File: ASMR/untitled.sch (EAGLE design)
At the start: 60 parts, among them J1 U.FL-R-SMT(01), J3 2172034-1, J4 POWER_JACKSLT, Q1 MMBT3904, Q2 MMBT3904, Q3 12MHz, Q4 MC-306, U2 DS1307Z+, U3 MAX3444EASA, U4 AMS1117, U5 MAX232CSE, X1 MSTBA2

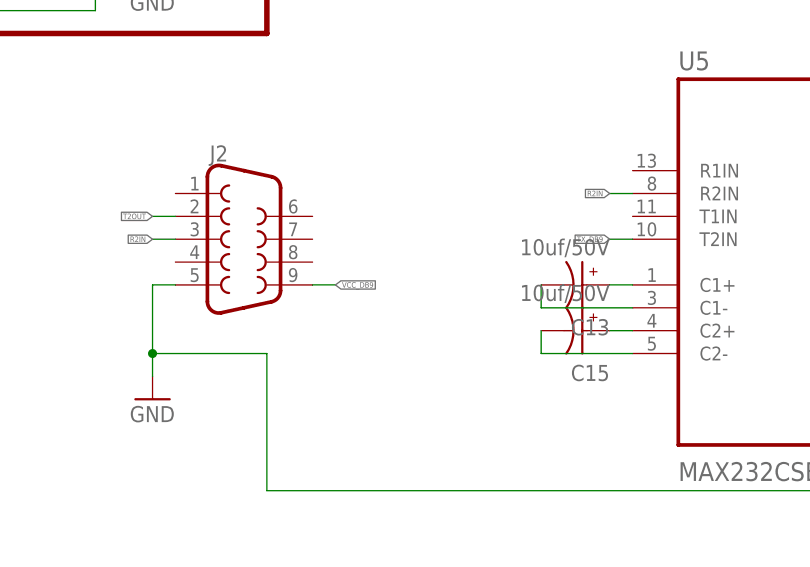
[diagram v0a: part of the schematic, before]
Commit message: penambahan komponen
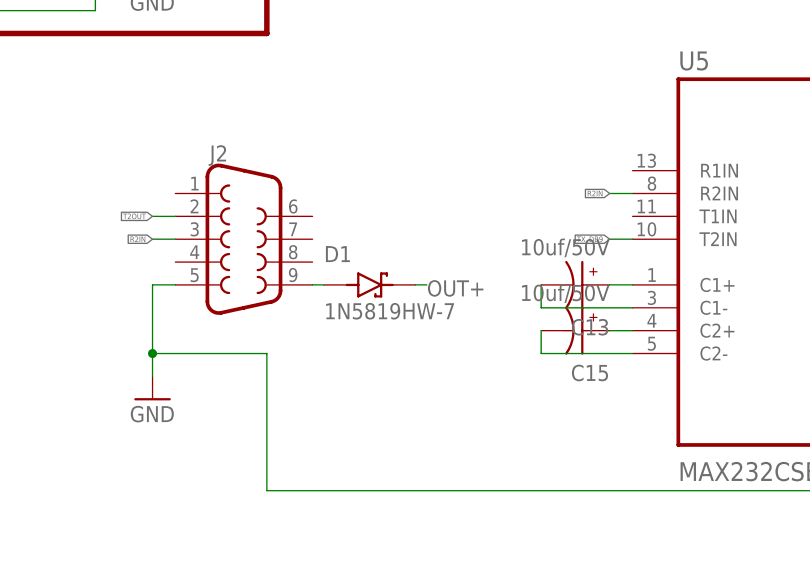
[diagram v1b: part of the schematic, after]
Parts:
- added D1: 1N5819HW-7, 1N5819HW-7:1N5819HW-7
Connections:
- new net N$20: D1.A, J2.9
- net OUT+: now also D1.K
- net VCC_DB9: no longer J2.9
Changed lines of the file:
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@@
 <part name="J1" library="U.FL-R-SMT_01_" deviceset="U.FL-R-SMT(01)" device=""/>
 <part name="JP3" library="pinhead" library_urn="urn:adsk.eagle:library:325" deviceset="PINHD-1X3" device="" package3d_urn="urn:adsk.eagle:package:22458/2"/>
+<part name="D1" library="1N5819HW-7" deviceset="1N5819HW-7" device=""/>
 </parts>
 <sheets>
@@
 <attribute name="NAME" x="85.09" y="121.285" size="1.778" layer="95"/>
 <attribute name="VALUE" x="85.09" y="107.95" size="1.778" layer="96"/>
+</instance>
+<instance part="D1" gate="G$1" x="59.69" y="-63.5" smashed="yes">
+<attribute name="NAME" x="54.61" y="-60.96" size="1.778" layer="95"/>
+<attribute name="VALUE" x="54.61" y="-67.31" size="1.778" layer="96"/>
 </instance>
 </instances>
@@
 <label x="-43.18" y="-30.48" size="1.778" layer="95" rot="R90" xref="yes"/>
 </segment>
+<segment>
+<pinref part="D1" gate="G$1" pin="K"/>
+<wire x1="64.77" y1="-63.5" x2="66.04" y2="-63.5" width="0.1524" layer="91"/>
+<label x="66.04" y="-64.77" size="1.778" layer="95"/>
+</segment>
 </net>
 <net name="MISO_HSPI" class="0">
@@
 </net>
 <net name="VCC_DB9" class="0">
-<segment>
-<pinref part="J2" gate="G$1" pin="9"/>
-<wire x1="53.34" y1="-63.5" x2="55.88" y2="-63.5" width="0.1524" layer="91"/>
-<label x="55.88" y="-63.5" size="0.6096" layer="95" xref="yes"/>
-</segment>
 <segment>
 <pinref part="D6" gate="G$1" pin="K"/>
@@
 </segment>
 </net>
+<net name="N$20" class="0">
+<segment>
+<pinref part="J2" gate="G$1" pin="9"/>
+<pinref part="D1" gate="G$1" pin="A"/>
+<wire x1="53.34" y1="-63.5" x2="54.61" y2="-63.5" width="0.1524" layer="91"/>
+</segment>
+</net>
